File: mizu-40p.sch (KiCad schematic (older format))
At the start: 118 parts

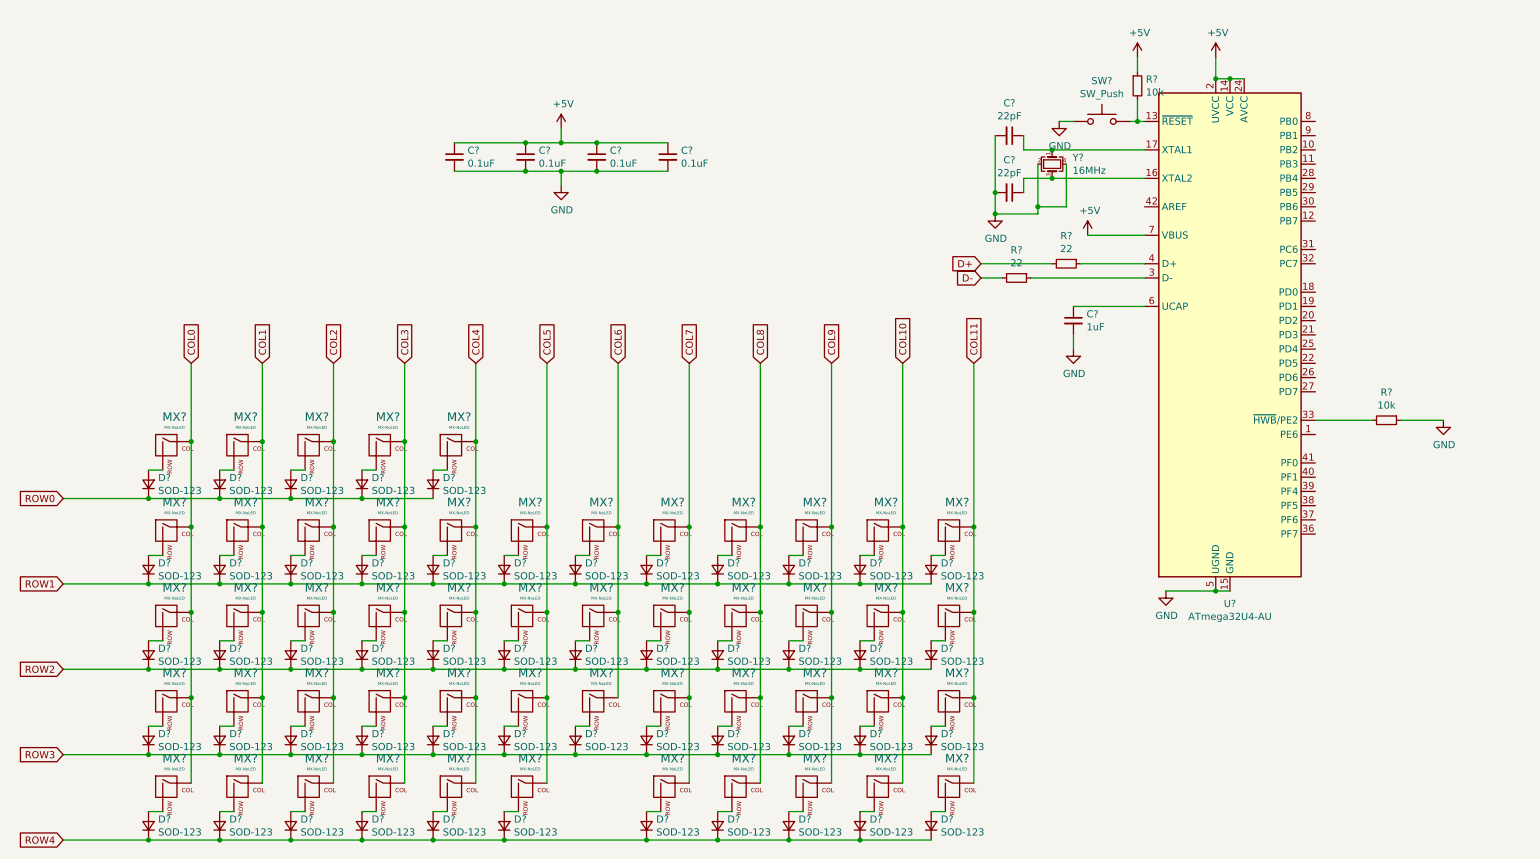
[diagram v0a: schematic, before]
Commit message: Change layout
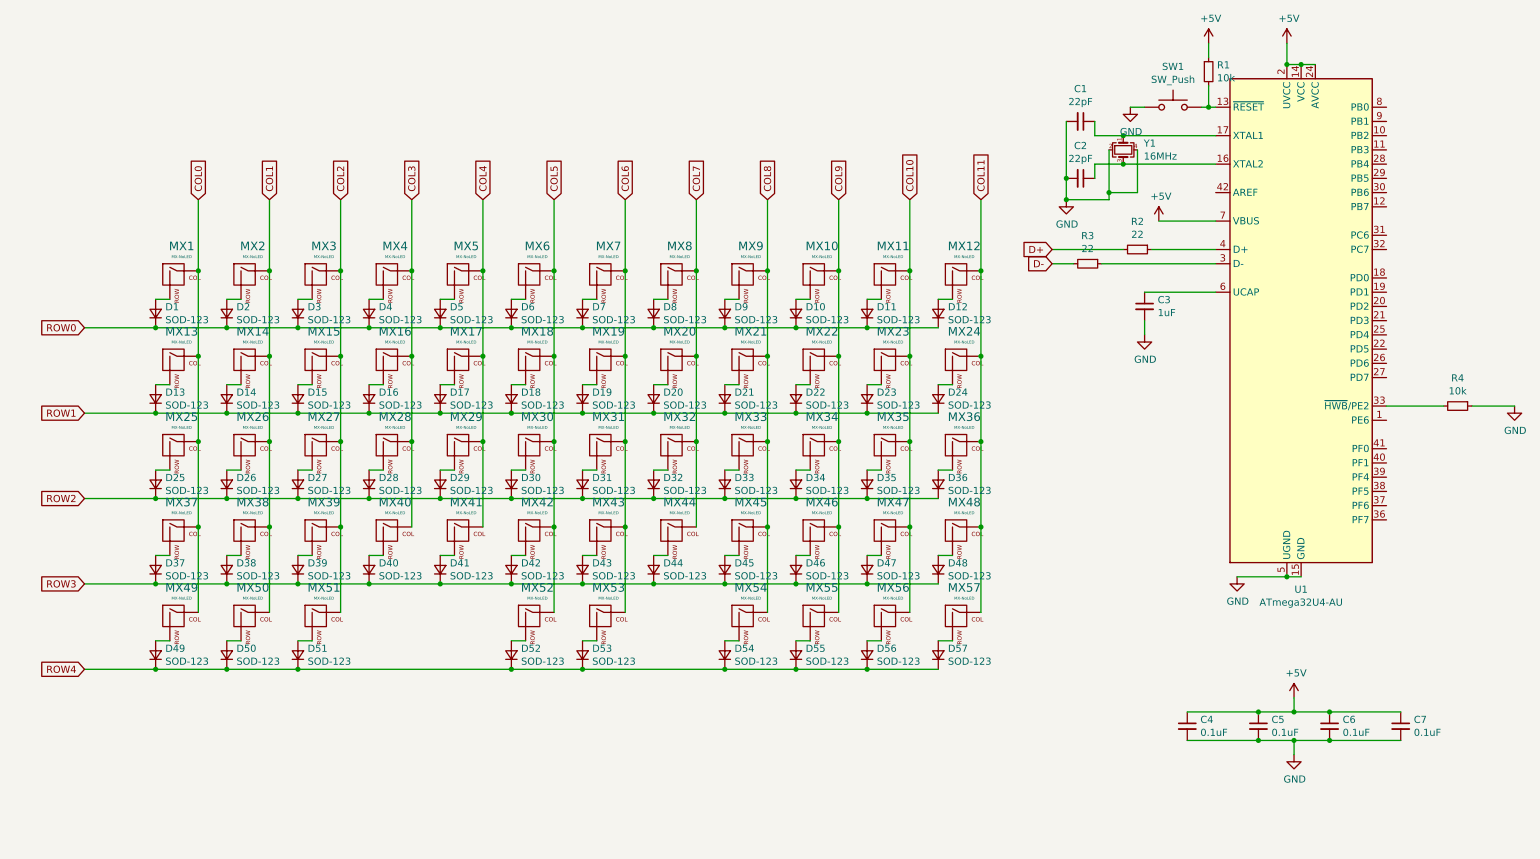
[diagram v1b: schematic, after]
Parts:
- removed D? (x45): SOD-123, symbol Device:D_Small
- removed MX? (x45): MX-NoLED, symbol MX_Alps_Hybrid:MX-NoLED
- added D1, D10, D11, D12, D13, D14, D15, D16, D17, D18, D19, D2, D20, D21, D22, D23, D24, D25, D26, D27, D28, D29, D3, D30, D31, D32, D33, D34, D35, D36, D37, D38, D39, D4, D40, D41, D42, D43, D44, D45, D46, D47, D48, D49, D5, D50, D6, D7, D8, D9: SOD-123, Diode_SMD:D_SOD-123, symbol Device:D_Small
- added MX1, MX10, MX11, MX12, MX13, MX14, MX15, MX16, MX17, MX18, MX19, MX2, MX20, MX21, MX22, MX23, MX24, MX25, MX26, MX27, MX28, MX29, MX3, MX30, MX31, MX32, MX33, MX34, MX35, MX36, MX37, MX38, MX39, MX4, MX40, MX41, MX42, MX43, MX44, MX45, MX46, MX47, MX48, MX49, MX5, MX50, MX6, MX7, MX8, MX9: MX-NoLED, MX_Alps_Hybrid:MX-1U-NoLED, symbol MX_Alps_Hybrid:MX-NoLED
- C1, C2, C3, C4, C5, C6, C7: renamed from C?; footprint (none) -> Capacitor_SMD:C_0805_2012Metric
- D51, D52, D53, D54, D55, D56, D57: renamed from D?; footprint (none) -> Diode_SMD:D_SOD-123
- MX51, MX52, MX53, MX54, MX55, MX56, MX57: renamed from MX?; footprint (none) -> MX_Alps_Hybrid:MX-1U-NoLED
- R1, R2, R3, R4: renamed from R?; footprint (none) -> Resistor_SMD:R_0805_2012Metric
- SW1: renamed from SW?; footprint (none) -> random-keyboard-parts:SKQG-1155865
- gave numbers to parts that had none: 2
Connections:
- net COL0: now also MX1.1 (COL), MX13.1 (COL), MX25.1 (COL), MX37.1 (COL), MX49.1 (COL); no longer MX51.1 (COL)
- net COL1: now also MX14.1 (COL), MX2.1 (COL), MX26.1 (COL), MX38.1 (COL), MX50.1 (COL)
- net COL10: now also MX11.1 (COL), MX23.1 (COL), MX35.1 (COL), MX47.1 (COL)
- net COL11: now also MX12.1 (COL), MX24.1 (COL), MX36.1 (COL), MX48.1 (COL)
- net COL2: now also MX51.1 (COL), MX15.1 (COL), MX27.1 (COL), MX3.1 (COL), MX39.1 (COL)
- net COL3: now also MX16.1 (COL), MX28.1 (COL), MX4.1 (COL), MX40.1 (COL); no longer MX52.1 (COL)
- net COL4: now also MX17.1 (COL), MX29.1 (COL), MX41.1 (COL), MX5.1 (COL); no longer MX53.1 (COL)
- net COL5: now also MX52.1 (COL), MX18.1 (COL), MX30.1 (COL), MX42.1 (COL), MX6.1 (COL)
- net COL6: now also MX53.1 (COL), MX19.1 (COL), MX31.1 (COL), MX43.1 (COL), MX7.1 (COL)
- net COL7: now also MX20.1 (COL), MX32.1 (COL), MX44.1 (COL), MX8.1 (COL)
- net COL8: now also MX21.1 (COL), MX33.1 (COL), MX45.1 (COL), MX9.1 (COL)
- net COL9: now also MX10.1 (COL), MX22.1 (COL), MX34.1 (COL), MX46.1 (COL)
- net ROW0: now also D1.1 (K), D10.1 (K), D11.1 (K), D12.1 (K), D2.1 (K), D3.1 (K), D4.1 (K), D5.1 (K), D6.1 (K), D7.1 (K), D8.1 (K), D9.1 (K)
- net ROW1: now also D13.1 (K), D14.1 (K), D15.1 (K), D16.1 (K), D17.1 (K), D18.1 (K), D19.1 (K), D20.1 (K), D21.1 (K), D22.1 (K), D23.1 (K), D24.1 (K)
- net ROW2: now also D25.1 (K), D26.1 (K), D27.1 (K), D28.1 (K), D29.1 (K), D30.1 (K), D31.1 (K), D32.1 (K), D33.1 (K), D34.1 (K), D35.1 (K), D36.1 (K)
- net ROW3: now also D37.1 (K), D38.1 (K), D39.1 (K), D40.1 (K), D41.1 (K), D42.1 (K), D43.1 (K), D44.1 (K), D45.1 (K), D46.1 (K), D47.1 (K), D48.1 (K)
- net ROW4: now also D49.1 (K), D50.1 (K)
- new net: D50.2 (A), MX50.2 (ROW)
- new net: D49.2 (A), MX49.2 (ROW)
- new net: D39.2 (A), MX39.2 (ROW)
- new net: D40.2 (A), MX40.2 (ROW)
- new net: D41.2 (A), MX41.2 (ROW)
- new net: D42.2 (A), MX42.2 (ROW)
- new net: D43.2 (A), MX43.2 (ROW)
- new net: D44.2 (A), MX44.2 (ROW)
- new net: D45.2 (A), MX45.2 (ROW)
- new net: D46.2 (A), MX46.2 (ROW)
- new net: D47.2 (A), MX47.2 (ROW)
- new net: D48.2 (A), MX48.2 (ROW)
- new net: D38.2 (A), MX38.2 (ROW)
- new net: D37.2 (A), MX37.2 (ROW)
- new net: D27.2 (A), MX27.2 (ROW)
- new net: D28.2 (A), MX28.2 (ROW)
- new net: D29.2 (A), MX29.2 (ROW)
- new net: D30.2 (A), MX30.2 (ROW)
- new net: D31.2 (A), MX31.2 (ROW)
- new net: D32.2 (A), MX32.2 (ROW)
- new net: D33.2 (A), MX33.2 (ROW)
- new net: D34.2 (A), MX34.2 (ROW)
- new net: D35.2 (A), MX35.2 (ROW)
- new net: D36.2 (A), MX36.2 (ROW)
- new net: D26.2 (A), MX26.2 (ROW)
- new net: D25.2 (A), MX25.2 (ROW)
- new net: D15.2 (A), MX15.2 (ROW)
- new net: D16.2 (A), MX16.2 (ROW)
- new net: D17.2 (A), MX17.2 (ROW)
- new net: D18.2 (A), MX18.2 (ROW)
- new net: D19.2 (A), MX19.2 (ROW)
- new net: D20.2 (A), MX20.2 (ROW)
- new net: D21.2 (A), MX21.2 (ROW)
- new net: D22.2 (A), MX22.2 (ROW)
- new net: D23.2 (A), MX23.2 (ROW)
- new net: D24.2 (A), MX24.2 (ROW)
- new net: D14.2 (A), MX14.2 (ROW)
- new net: D13.2 (A), MX13.2 (ROW)
- new net: D3.2 (A), MX3.2 (ROW)
- new net: D4.2 (A), MX4.2 (ROW)
- new net: D5.2 (A), MX5.2 (ROW)
- new net: D6.2 (A), MX6.2 (ROW)
- new net: D7.2 (A), MX7.2 (ROW)
- new net: D8.2 (A), MX8.2 (ROW)
- new net: D9.2 (A), MX9.2 (ROW)
- new net: D10.2 (A), MX10.2 (ROW)
- new net: D11.2 (A), MX11.2 (ROW)
- new net: D12.2 (A), MX12.2 (ROW)
- new net: D2.2 (A), MX2.2 (ROW)
- new net: D1.2 (A), MX1.2 (ROW)
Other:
- moved on the sheet: C1, C2, C3, C4, C5, C6, C7, D51, D52, D53, D54, D55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
